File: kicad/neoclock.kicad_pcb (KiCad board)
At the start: 2 copper layers, 28.1 x 42.7 mm, 22 parts, among them CON1 2.1mm 5V, IC1 ATMEGA328P-A, K1 NEOPIXEL, P1 ICSP, SW1 HOUR, SW2 MINUTE, U1 DS1307, X1 16Mhz, X2 32.768kHz

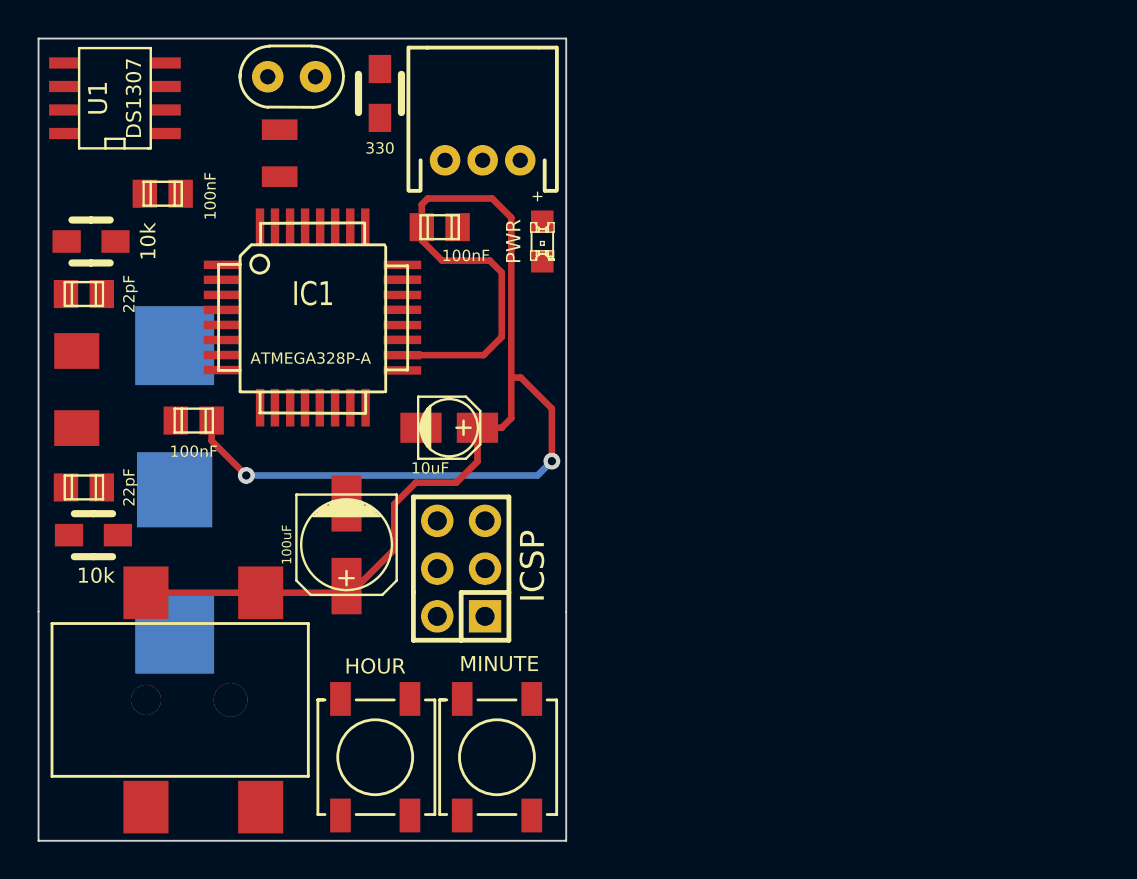
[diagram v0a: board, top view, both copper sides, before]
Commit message: updated qfn board
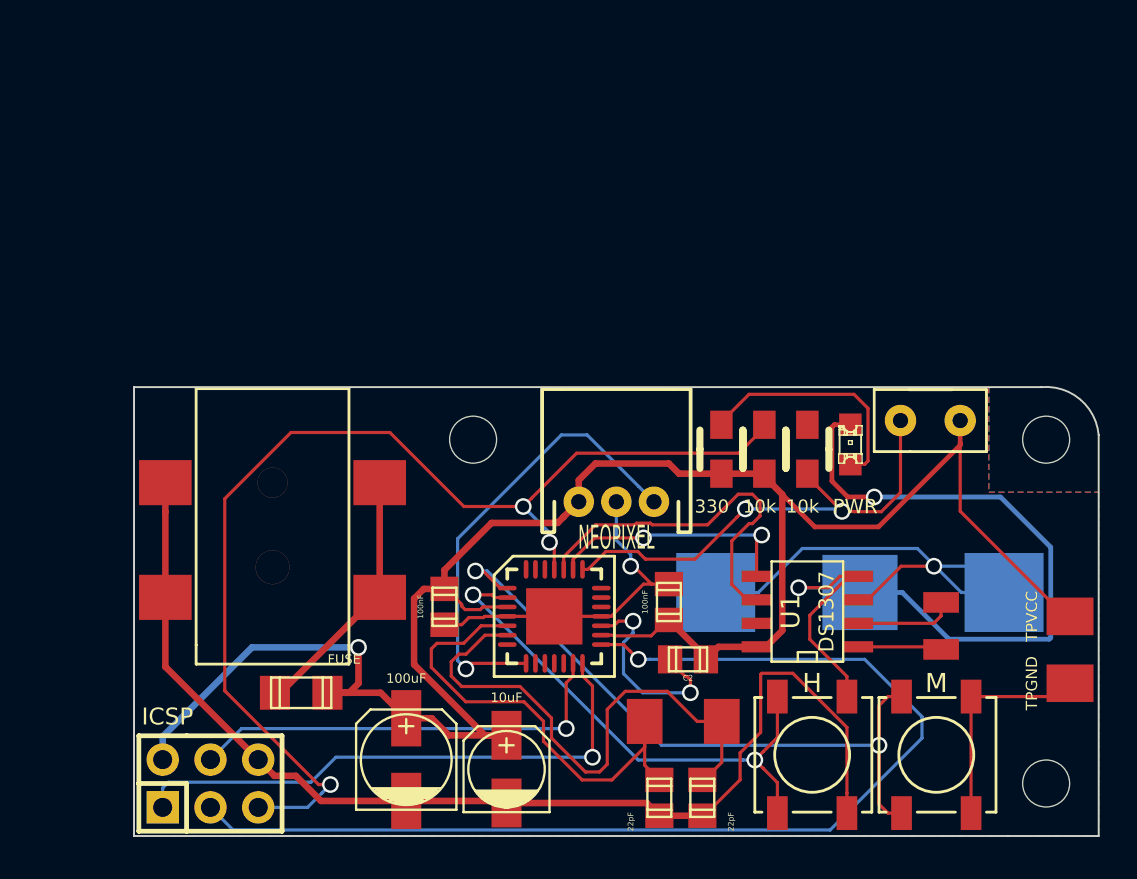
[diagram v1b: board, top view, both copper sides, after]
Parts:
- added F1: FUSE, synic:1206_polyfuse, F.Cu at (33.0, 51.3)
- added MH: MountingHole_2-5mm_RevA_Date21Jun2010, Mounting_Holes:MountingHole_2-5mm, F.Cu at (72.6, 56.1)
- added MH: MountingHole_2-5mm_RevA_Date21Jun2010, Mounting_Holes:MountingHole_2-5mm, F.Cu at (42.2, 37.8)
- added MH1: MountingHole_2-5mm_RevA_Date21Jun2010, Mounting_Holes:MountingHole_2-5mm, F.Cu at (72.6, 37.8)
- added TP1: TPGND, synicpretty:TESTPOINT, F.Cu at (73.9, 50.8)
- added TP2: TPVCC, TESTPOINT, F.Cu at (73.9, 47.2)
- C4: footprint Capacitors_SMD:c_elec_3x5.3 -> Capacitors_SMD:c_elec_4x5.3
- CON1: footprint synic:BARREL_JACK_SMD -> BARREL_JACK_SMD
- IC1: value ATMEGA328P-A -> ATMEGA328P-MM; footprint SMD_Packages:TQFP32 -> SMD_Packages:QFN28
- PHOTOR1: footprint synic:PHOTORESISTOR -> PHOTORESISTOR
- SW1: value HOUR -> H
- SW2: value MINUTE -> M
- moved U1 45.8 mm to (59.9, 47.0)
- moved X2 43.2 mm to (67.1, 47.8)
- moved C5 40.7 mm to (52.1, 56.9), turned to 270 degrees
- moved PHOTOR1 38.6 mm to (66.5, 36.8)
- moved R3 38.2 mm to (59.9, 38.4), turned to 90 degrees
- moved R2 37.5 mm to (57.7, 38.4), turned to 90 degrees
- moved BT1 36.9 mm to (62.7, 46.0), turned to 0 degrees
- moved C6 36.8 mm to (54.4, 56.9), turned to 270 degrees
- moved X1 36.8 mm to (53.3, 52.8), turned to 0 degrees
- moved C7 34.6 mm to (52.6, 46.5), turned to 90 degrees
- moved C2 26.5 mm to (53.6, 49.5), turned to 180 degrees
- moved R1 26.2 mm to (55.4, 38.4), turned to 90 degrees
- moved SW2 23.4 mm to (66.8, 54.6)
- moved SW1 23.2 mm to (60.2, 54.6)
- moved IC1 20.4 mm to (46.5, 47.2)
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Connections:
- CON1 pad 1: VCC -> Net-(CON1-Pad1)
- IC1 pad 16: Net-(IC1-Pad16) -> VCC
- IC1 pad 17: Net-(IC1-Pad17) -> Net-(C2-Pad1)
- IC1 pad 18: VCC -> GND
- IC1 pad 20: Net-(C2-Pad1) -> Net-(IC1-Pad20)
- IC1 pad 21: GND -> Net-(IC1-Pad21)
- IC1 pad 23: Net-(IC1-Pad23) -> I2CSDA
- IC1 pad 24: Net-(IC1-Pad24) -> I2CSCL
- IC1 pad 27: I2CSDA -> Net-(IC1-Pad27)
- IC1 pad 28: I2CSCL -> Net-(IC1-Pad28)
- IC1 pad 29: Net-(IC1-Pad29) -> GND
- IC1 pad 3: GND -> VCC
- IC1 pad 4: VCC -> GND
- IC1 pad 5: GND -> Net-(C5-Pad2)
- IC1 pad 6: VCC -> Net-(C6-Pad2)
- IC1 pad 7: Net-(C5-Pad2) -> Net-(IC1-Pad7)
- IC1 pad 8: Net-(C6-Pad2) -> Net-(IC1-Pad8)
- K1 pad 3: Net-(IC1-Pad10) -> Net-(IC1-Pad8)
- P1 pad 1: Net-(IC1-Pad16) -> Net-(IC1-Pad14)
- P1 pad 3: Net-(IC1-Pad17) -> Net-(IC1-Pad15)
- P1 pad 4: Net-(IC1-Pad15) -> Net-(IC1-Pad13)
- P1 pad 5: Net-(IC1-Pad29) -> Net-(IC1-Pad25)
- PHOTOR1 pad 2: Net-(IC1-Pad26) -> Net-(IC1-Pad22)
- R2 pad 2: Net-(IC1-Pad29) -> Net-(IC1-Pad25)
- R3 pad 1: Net-(IC1-Pad26) -> Net-(IC1-Pad22)
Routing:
- net GND: track 0.00 -> 139.1 mm, vias 0 -> 3
- net Net-(IC1-Pad15): track 0.00 -> 60.2 mm, vias 0 -> 1
- net Net-(IC1-Pad25): track 0.00 -> 60.0 mm, vias 0 -> 3
- net Net-(IC1-Pad1): track 0.00 -> 35.4 mm, vias 0 -> 2
- net Net-(IC1-Pad14): track 0.00 -> 29.8 mm, vias 0 -> 1
- net Net-(C6-Pad2): track 0.00 -> 29.2 mm
- net VCC: track 83.6 -> 112.7 mm, vias 2 -> 1
- net Net-(IC1-Pad2): track 0.00 -> 27.7 mm, vias 0 -> 2
- net Net-(BT1-Pad1): track 0.00 -> 26.4 mm, vias 0 -> 1
- net Net-(IC1-Pad22): track 0.00 -> 25.7 mm, vias 0 -> 2
- net Net-(C5-Pad2): track 0.00 -> 25.5 mm
- net Net-(IC1-Pad8): track 0.00 -> 24.6 mm, vias 0 -> 1
- net Net-(IC1-Pad13): track 0.00 -> 23.2 mm, vias 0 -> 1
- net I2CSCL: track 0.00 -> 19.5 mm
- net Net-(CON1-Pad1): track 0.00 -> 13.8 mm
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- added copper zone on B.Cu, net GND
- added copper zone on F.Cu, net GND
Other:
- board size 28.1 x 42.7 mm -> 51.3 x 23.9 mm
- net class POWER removed
- net class PWR added: clearance 0.254, trace_width 0.35, via_dia 0.889, via_drill 0.635
- rule trace_min: 0.254 -> 0.17
- board text added: "NeoClock v5 arolsen@gmail.com"
- board text removed: "+"

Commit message: commit latest changes for orsonz
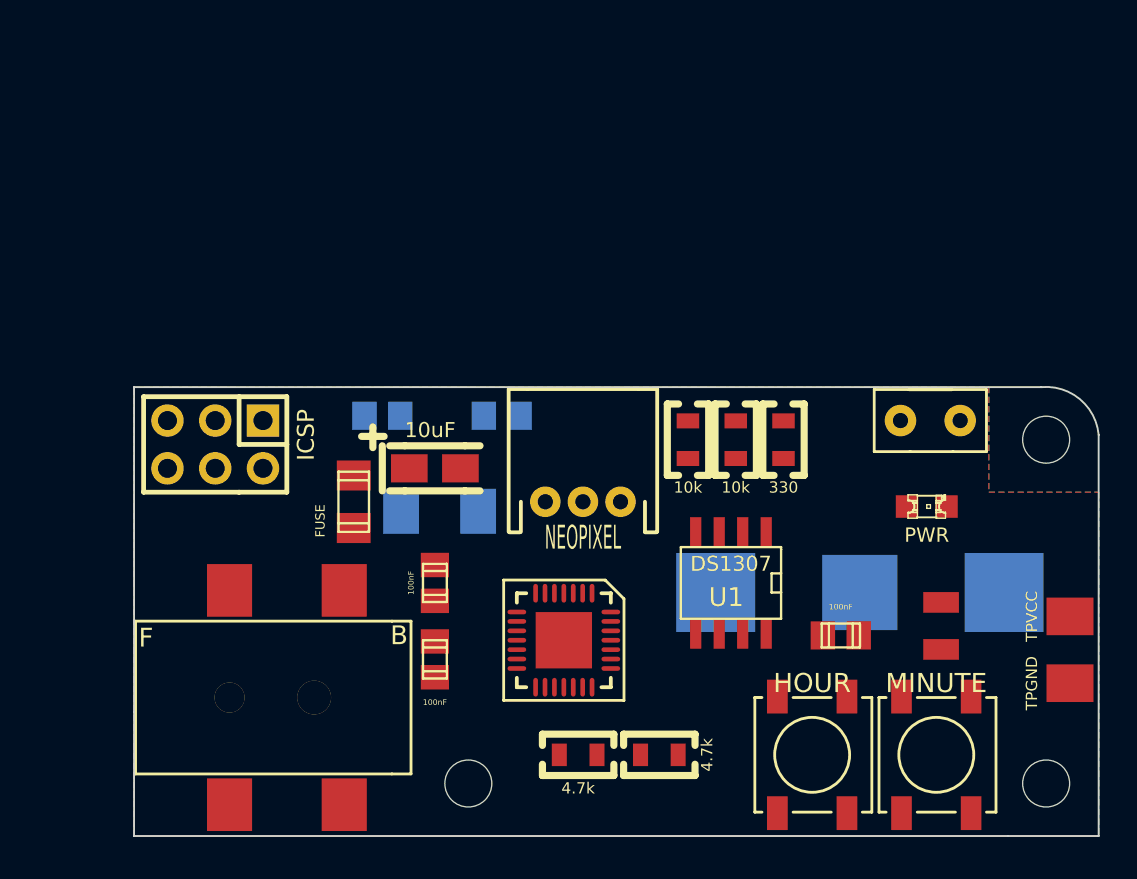
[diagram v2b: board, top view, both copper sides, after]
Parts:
- removed C3: 100uF, Capacitors_SMD:c_elec_5x5.3
- added R4: 4.7k, Resistors_SMD:Resistor_SMD0805_ReflowWave, F.Cu at (52.1, 54.6)
- added R5: 4.7k, Resistors_SMD:Resistor_SMD0805_ReflowWave, F.Cu at (47.8, 54.6)
- C4: footprint Capacitors_SMD:c_elec_4x5.3 -> Capacitors_Tantalum_SMD:TantalC_SizeA_EIA-3216_Reflow
- C5, C6, X1: moved to B.Cu
- R1, R2, R3: footprint Resistors_SMD:Resistor_SMD0805_HandSoldering -> Resistors_SMD:Resistor_SMD0805_ReflowWave
- SW1: value H -> HOUR
- SW2: value M -> MINUTE
- moved C6 26.5 mm to (37.3, 36.6), turned to 0 degrees
- moved C5 22.0 mm to (43.7, 36.6), turned to 180 degrees
- moved MH 18.3 mm to (41.9, 56.1)
- moved P1 18.0 mm to (28.4, 38.1), turned to 180 degrees
- moved X1 17.1 mm to (40.4, 41.7), turned to 180 degrees
- moved C4 16.4 mm to (40.1, 39.4), turned to 0 degrees
- moved C2 13.5 mm to (40.1, 49.5), turned to 90 degrees
- moved CON1 11.7 mm to (29.2, 51.6), turned to 0 degrees
- moved F1 10.5 mm to (35.8, 41.1), turned to 270 degrees
- moved C7 9.32 mm to (61.7, 48.3), turned to 0 degrees
- moved D1 5.24 mm to (66.3, 41.4), turned to 0 degrees
- moved U1 4.34 mm to (55.9, 45.5), turned to 180 degrees
- moved R2 4.10 mm to (53.6, 37.8)
- moved R3 3.84 mm to (56.1, 37.8)
- moved R1 3.34 mm to (58.7, 37.8)
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- renumbered MH to MH5
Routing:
- net GND: track 139.1 -> 0.00 mm, vias 3 -> 0
- net VCC: track 112.7 -> 0.00 mm, vias 1 -> 0
- net Net-(IC1-Pad15): track 60.2 -> 0.00 mm, vias 1 -> 0
- net Net-(IC1-Pad25): track 60.0 -> 0.00 mm, vias 3 -> 0
- net Net-(IC1-Pad1): track 35.4 -> 0.00 mm, vias 2 -> 0
- net Net-(IC1-Pad14): track 29.8 -> 0.00 mm, vias 1 -> 0
- net Net-(C6-Pad2): track 29.2 -> 0.00 mm
- net Net-(IC1-Pad2): track 27.7 -> 0.00 mm, vias 2 -> 0
- net Net-(BT1-Pad1): track 26.4 -> 0.00 mm, vias 1 -> 0
- net Net-(IC1-Pad22): track 25.7 -> 0.00 mm, vias 2 -> 0
- net Net-(C5-Pad2): track 25.5 -> 0.00 mm
- net Net-(IC1-Pad8): track 24.6 -> 0.00 mm, vias 1 -> 0
- net Net-(IC1-Pad13): track 23.2 -> 0.00 mm, vias 1 -> 0
- net I2CSCL: track 19.5 -> 0.00 mm
- net Net-(CON1-Pad1): track 13.8 -> 0.00 mm
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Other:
- net class LRGPWR added: clearance 0.254, trace_width 0.4, via_dia 0.889, via_drill 0.635

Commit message: woot
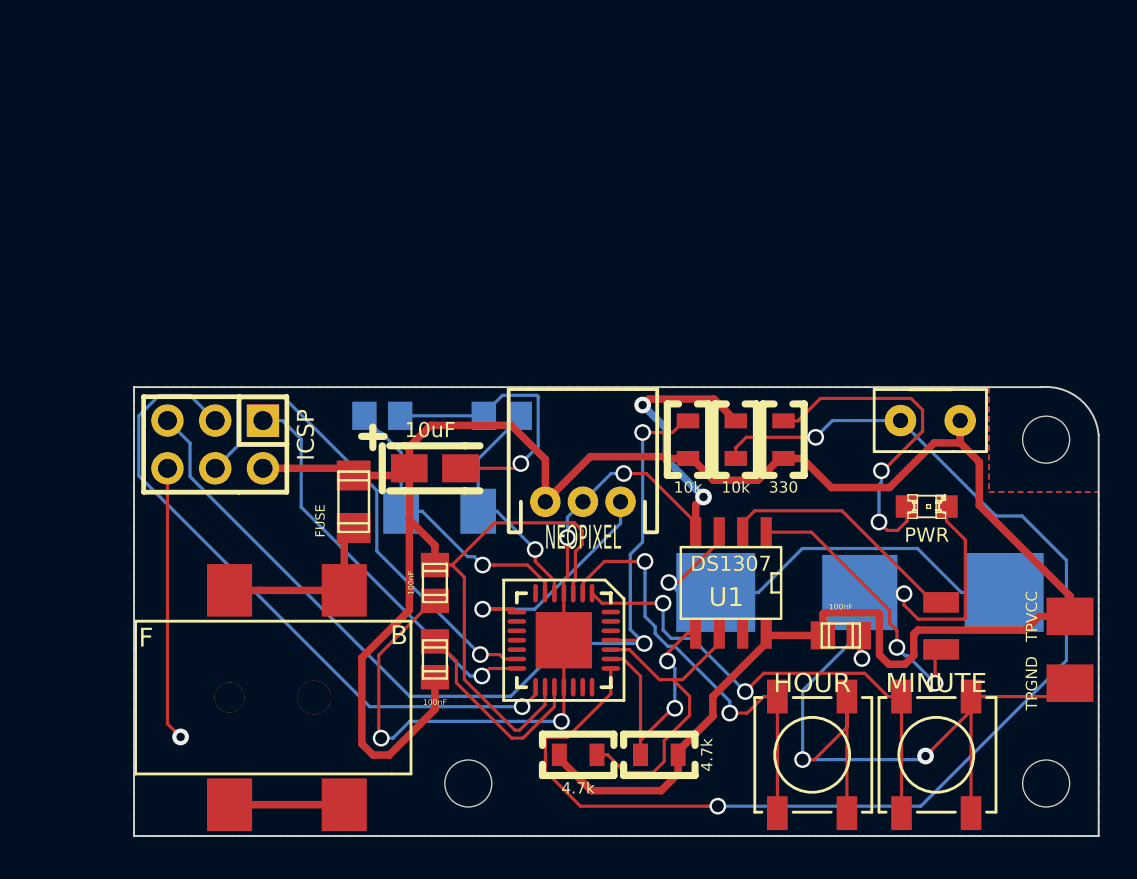
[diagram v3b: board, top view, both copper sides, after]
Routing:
- net GND: track 0.00 -> 150.0 mm, vias 0 -> 12
- net VCC: track 0.00 -> 148.2 mm
- net Net-(IC1-Pad22): track 0.00 -> 66.4 mm, vias 0 -> 2
- net Net-(IC1-Pad25): track 0.00 -> 50.0 mm, vias 0 -> 2
- net Net-(IC1-Pad15): track 0.00 -> 35.1 mm, vias 0 -> 1
- net Net-(IC1-Pad13): track 0.00 -> 26.6 mm, vias 0 -> 1
- net Net-(IC1-Pad1): track 0.00 -> 26.6 mm, vias 0 -> 2
- net Net-(BT1-Pad1): track 0.00 -> 24.1 mm, vias 0 -> 1
- net Net-(IC1-Pad2): track 0.00 -> 23.6 mm, vias 0 -> 2
- net Net-(IC1-Pad14): track 0.00 -> 21.4 mm, vias 0 -> 1
- net Net-(D1-Pad1): track 0.00 -> 17.8 mm, vias 0 -> 2
- net I2CSCL: track 0.00 -> 17.2 mm
- net Net-(C6-Pad2): track 0.00 -> 15.7 mm, vias 0 -> 1
- net Net-(U1-Pad1): track 0.00 -> 15.2 mm, vias 0 -> 2
- net I2CSDA: track 0.00 -> 13.7 mm, vias 0 -> 2
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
